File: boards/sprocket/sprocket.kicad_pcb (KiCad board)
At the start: 2 copper layers, 47 x 15 mm, 14 parts, among them U1 STM32G031F8P6

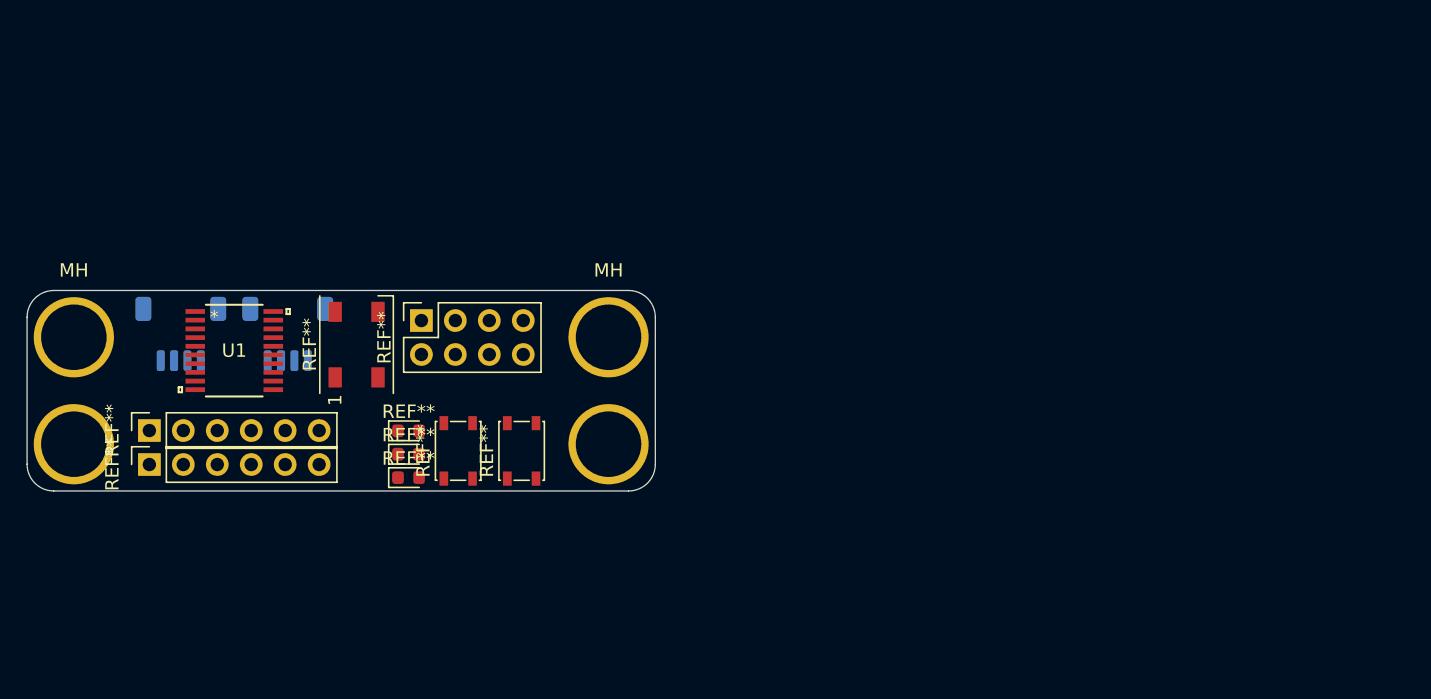
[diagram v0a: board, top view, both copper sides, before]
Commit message: I don't know what this branch is
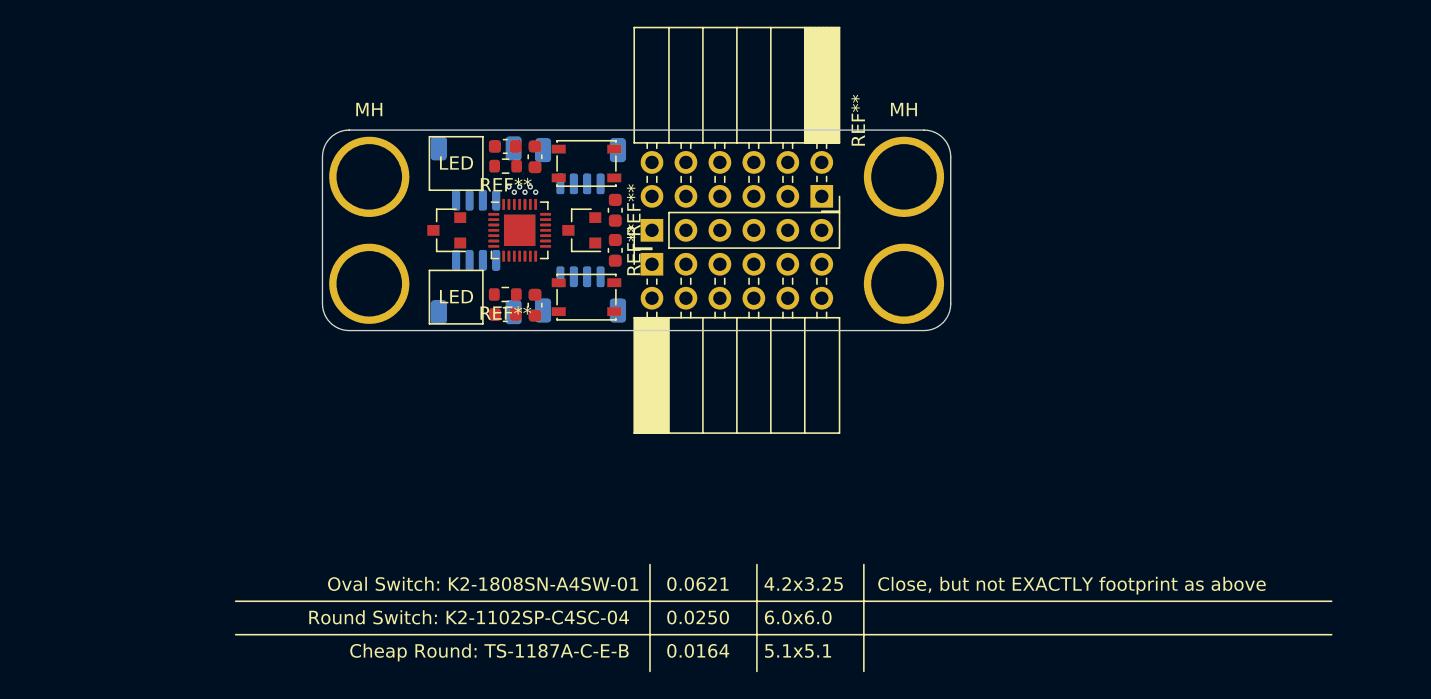
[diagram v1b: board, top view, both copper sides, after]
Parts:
- removed the MH at (144.0, 104.0)
- removed the MH at (104.0, 104.0)
- removed the REF** at (125.2, 104.5)
- removed the REF** at (120.0, 103.8)
- removed the REF** at (112.0, 103.8)
- removed the REF** at (129.0, 111.0)
- removed the REF** at (129.0, 112.8)
- removed the REF** at (129.0, 114.5)
- removed the REF** at (132.8, 112.5)
- removed the REF** at (137.5, 112.5)
- removed the REF** at (130.0, 102.8)
- removed the REF** at (109.7, 113.5)
- removed the REF** at (109.7, 111.0)
- removed U1: STM32G031F8P6, footprints:STM32G031F8P6
- added MH: brick-1x2, brick-4_9id-6_0od:brick-1x2, F.Cu at (126.1, 92.0)
- added MH: brick-1x2, brick-4_9id-6_0od:brick-1x2, F.Cu at (166.1, 92.0)
- added REF**: C_0603_1608Metric, Capacitor_SMD:C_0603_1608Metric, F.Cu at (138.5, 101.6)
- added REF**: SW_SPST_PTS810, Button_Switch_SMD:SW_SPST_PTS810, F.Cu at (142.3, 101.0)
- added REF**: SW_SPST_PTS810, Button_Switch_SMD:SW_SPST_PTS810, F.Cu at (142.3, 91.0)
- added REF**: UQFN-28-1EP_4x4mm_P0.4mm_EP2.35x2.35mm, Package_DFN_QFN:UQFN-28-1EP_4x4mm_P0.4mm_EP2.35x2.35mm, F.Cu at (137.3, 96.0)
- added REF**: SOT-23, Package_TO_SOT_SMD:SOT-23, F.Cu at (142.0, 96.0)
- added REF**: JST_SH_BM04B-SRSS-TB_1x04-1MP_P1.00mm_Vertical, Connector_JST:JST_SH_BM04B-SRSS-TB_1x04-1MP_P1.00mm_Vertical, B.Cu at (141.9, 100.8)
- added REF**: JST_SH_BM04B-SRSS-TB_1x04-1MP_P1.00mm_Vertical, Connector_JST:JST_SH_BM04B-SRSS-TB_1x04-1MP_P1.00mm_Vertical, B.Cu at (141.9, 91.2)
- added REF**: JST_SH_SM04B-SRSS-TB_1x04-1MP_P1.00mm_Horizontal, Connector_JST:JST_SH_SM04B-SRSS-TB_1x04-1MP_P1.00mm_Horizontal, B.Cu at (134.1, 100.2)
- added REF**: JST_SH_SM04B-SRSS-TB_1x04-1MP_P1.00mm_Horizontal, Connector_JST:JST_SH_SM04B-SRSS-TB_1x04-1MP_P1.00mm_Horizontal, B.Cu at (134.1, 91.8)
- added REF**: PinHeader_1x06_P2.54mm_Vertical, Connector_PinHeader_2.54mm:PinHeader_1x06_P2.54mm_Vertical, F.Cu at (147.2, 96.0)
- added REF**: PinSocket_2x06_P2.54mm_Horizontal, Connector_PinSocket_2.54mm:PinSocket_2x06_P2.54mm_Horizontal, F.Cu at (147.2, 98.5)
- added REF**: C_0603_1608Metric, Capacitor_SMD:C_0603_1608Metric, F.Cu at (138.5, 90.5)
- added REF**: PinSocket_2x06_P2.54mm_Horizontal, Connector_PinSocket_2.54mm:PinSocket_2x06_P2.54mm_Horizontal, F.Cu at (159.9, 93.5)
- added REF**: R_0603_1608Metric, Resistor_SMD:R_0603_1608Metric, F.Cu at (136.3, 100.8)
- added REF**: R_0603_1608Metric, Resistor_SMD:R_0603_1608Metric, F.Cu at (136.3, 91.2)
- added REF**: C_0603_1608Metric, Capacitor_SMD:C_0603_1608Metric, F.Cu at (144.5, 94.5)
- added REF**: C_0603_1608Metric, Capacitor_SMD:C_0603_1608Metric, F.Cu at (144.5, 97.5)
- added REF**: C_0603_1608Metric, Capacitor_SMD:C_0603_1608Metric, F.Cu at (136.3, 102.3)
- added REF**: C_0603_1608Metric, Capacitor_SMD:C_0603_1608Metric, F.Cu at (136.3, 89.7)
- added REF**: SOT-23, Package_TO_SOT_SMD:SOT-23, F.Cu at (131.9, 96.0)
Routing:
- net (no net): track 0.00 -> 0.25 mm, vias 0 -> 6
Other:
- rule trace_min: 0.2 -> 0.09
- rule via_min_drill: 0.3 -> 0.2
- board text added: "0.0164"
- board text added: "0.0250"
- board text added: "0.0621"
- board text added: "4.2x3.25"
- board text added: "5.1x5.1"
- board text added: "6.0x6.0"
- board text added: "Cheap Round: TS-1187A-C-E-B"
- board text added: "Close, but not EXACTLY footprint as above"
- board text added: "Digital Port"
- board text added: "GND"
- board text added: "GPIO port"
- board text added: "LED"
- board text added: "One Space Horizontal, maybe Vertical"
- board text added: "Oval Switch: K2-1808SN-A4SW-01"
- board text added: "Programming/Debugging Port"
- board text added: "RGB LED"
- board text added: "Round Switch: K2-1102SP-C4SC-04"
- board text added: "SCL"
- board text added: "SDA"
- board text added: "VCC"
